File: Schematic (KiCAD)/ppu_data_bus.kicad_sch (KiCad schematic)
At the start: 111 parts

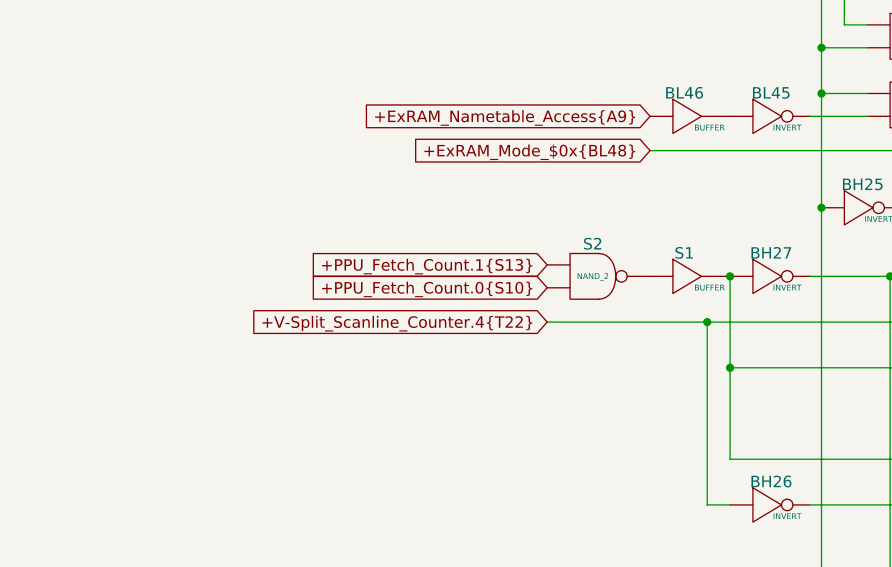
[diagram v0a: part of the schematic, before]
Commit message: Schematic and SVG Updates
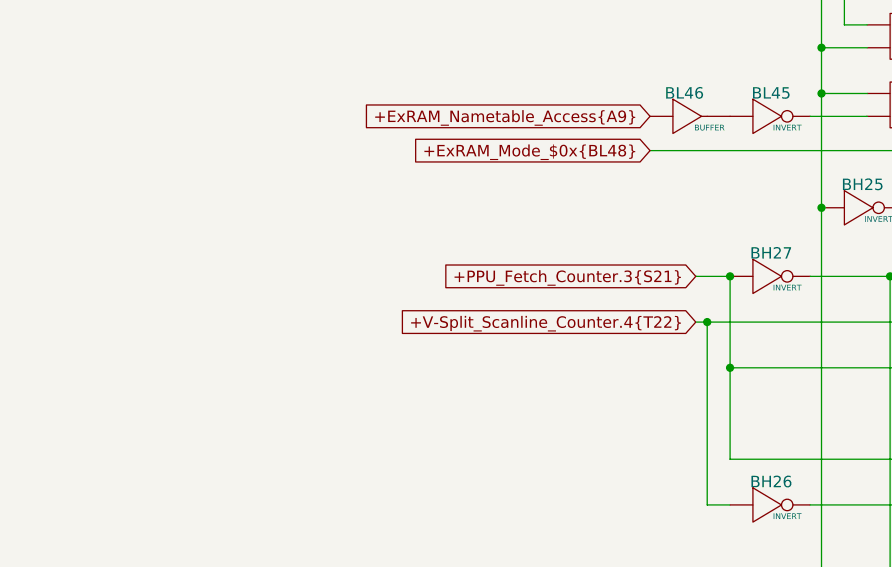
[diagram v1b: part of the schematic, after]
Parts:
- removed S1: BUFFER, symbol MMC5:BUFFER
- removed S2: NAND_2, symbol MMC5:NAND_2
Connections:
- net at BK24. (X): now also BK23. (X); no longer BK25. (X)
- net at BK23. (X): now also BL16. (X); no longer BK24. (X)
- net at BL14. (X): now also BL2. (X); no longer BK15. (X)
- net at BL45. (X): now also BL46. (X); no longer BL41. (X)
- net at BH21. (X): now also BH12. (X), BH4. (X); no longer BH22. (X)
- net at BK8. (X): now also BK7. (X); no longer BK9. (X)
- net at BK7. (X): now also BK15. (X), BK23. (X), BK31. (X), BK43. (X); no longer BK8. (X)
- net at BH19. (X): now also BH14. (X), BH6. (X); no longer BH20. (X)
- net at BH11. (X): now also BH12. (X); no longer BH13. (X)
- net at BL19. (X): now also BL7. (X); no longer BK35. (X)
- net at BL35. (X): now also BL29. (X); no longer BL40. (X)
- net at BL12. (X): now also BK1. (X); no longer BK7. (X)
- net at BK31. (X): now also BK32. (X); no longer BL18. (X)
- net at BK32. (X): now also BK33. (X); no longer BK31. (X)
- net at BK36. (X): now also BK35. (X); no longer BK37. (X)
- net at BH18. (X): now also BH22. (X), BH27. (X); no longer BH17. (X)
- net at BK28. (X): now also BK27. (X); no longer BK29. (X)
- net at BH2. (X): now also BH3. (X); no longer BH1. (X)
- net at BH3. (X): now also BH6. (X); no longer BH2. (X)
- net at BL16. (X): now also BL4. (X); no longer BK23. (X)
- net at BK11. (X): now also BK12. (X); no longer BL13. (X)
- net at BK12. (X): now also BK13. (X); no longer BK11. (X)
- net at BH10. (X): now also BH11. (X); no longer BH9. (X)
- net at BL15. (X): now also BK19. (X); no longer BL3. (X)
- net at BL17. (X): now also BL5. (X); no longer BK27. (X)
- net +PPU_Fetch_Counter.3{S21}: now reaches BH20. (X), BH24. (X), BH27. (X)
- net at BL37. (X): now also BL38. (X), BL42. (X); no longer BL36. (X)
- net at BK20. (X): now also BK19. (X); no longer BK21. (X)
- new net: BK24. (X), BK25. (X)
- new net: BL12. (X), BL13. (X), BL14. (X), BL15. (X), BL16. (X), BL17. (X), BL18. (X), BL19. (X), BL31. (X)
- new net: BK15. (X), BL14. (X)
- new net: BK10. (X), BK14. (X), BK18. (X), BK22. (X), BK26. (X), BK30. (X), BK34. (X), BK38. (X), BL39. (X)
- new net: BL41. (X), BL45. (X)
- new net: BL41. (X), BL42. (X)
- new net: BH21. (X), BH22. (X)
- new net: BK8. (X), BK9. (X)
- new net: BH19. (X), BH20. (X)
- new net: BK25. (X), BK26. (X)
- new net: BH13. (X), BH23. (X), BH5. (X)
- new net: BH11. (X), BH13. (X)
- new net: BK35. (X), BL19. (X)
- new net: BK10. (X), BK9. (X)
- new net: BL34. (X), BL35. (X), BL37. (X)
- new net: BL35. (X), BL40. (X)
- new net: BK7. (X), BL12. (X)
- new net: BK15. (X), BK23. (X), BK31. (X), BK42. (X), BK7. (X)
- new net: BK31. (X), BL18. (X)
- new net: BK37. (X), BK38. (X)
- new net: BK36. (X), BK37. (X)
- new net: BH18. (X), BH20. (X), BH26. (X)
- new net: BH18. (X), BH20. (X), BH22. (X), BH24. (X), BH25. (X)
- new net: BH17. (X), BH18. (X)
- new net: BH15. (X), BH17. (X), BH7. (X)
- new net: BH11. (X), BH15. (X)
- new net: BK29. (X), BK30. (X)
- new net: BK28. (X), BK29. (X)
- new net: BK11. (X), BK19. (X), BK27. (X), BK35. (X), BK40. (X)
- new net: BK39. (X), BK40. (X), BK42. (X)
- new net: BH1. (X), BH2. (X)
- new net: BK11. (X), BK19. (X), BK27. (X), BK35. (X), BK41. (X)
- new net: BK11. (X), BL13. (X)
- new net: BK21. (X), BK22. (X)
- new net: BK13. (X), BK14. (X)
- new net: BH10. (X), BH9. (X)
- new net: BK4. (X), BK5. (X)
- new net: BK2. (X), BK5. (X)
- new net: BL28. (X), BL29. (X), BL37. (X)
- new net: BL15. (X), BL3. (X)
- new net: BK27. (X), BL17. (X)
- new net: BK41. (X), BK43. (X), BK44. (X)
- new net: BL36. (X), BL37. (X)
- new net: BK20. (X), BK21. (X)
- new net: BK33. (X), BK34. (X)
- new net: BH11. (X), BH16. (X)
- new net: BH3. (X), BH5. (X)
- new net: BH3. (X), BH8. (X)
- new net: BH3. (X), BH4. (X)
- new net: BH3. (X), BH7. (X)
- new net: BK17. (X), BK18. (X)
- new net: BH11. (X), BH14. (X)
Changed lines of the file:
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@@
 	)
 	(junction
+		(at 170.18 86.36)
+		(diameter 0)
+		(color 0 0 0 0)
+	)
+	(junction
 		(at 224.79 86.36)
 		(diameter 0)
@@
 	)
 	(junction
-		(at 170.18 86.36)
-		(diameter 0)
-		(color 0 0 0 0)
-	)
-	(junction
 		(at 345.44 120.65)
 		(diameter 0)
@@
 	(wire
 		(pts
+			(xy 166.37 86.36) (xy 170.18 86.36)
+		)
+		(stroke
+			(width 0)
+			(type default)
+		)
+	)
+	(wire
+		(pts
 			(xy 271.78 25.4) (xy 274.32 25.4)
 		)
@@
 	(wire
 		(pts
-			(xy 149.86 91.44) (xy 167.64 91.44)
+			(xy 166.37 91.44) (xy 167.64 91.44)
 		)
 		(stroke
@@
 		)
 	)
-	(global_label "+PPU_Fetch_Count.0{S10}"
-		(shape input)
-		(at 149.86 87.63 180)
-		(fields_autoplaced yes)
-		(effects
-			(font
-				(size 1.27 1.27)
-			)
-			(justify right)
-		)
-		(property "Intersheetrefs" "${INTERSHEET_REFS}"
-			(at 121.7773 87.63 0)
-			(effects
-				(font
-					(size 1.27 1.27)
-				)
-				(justify right)
-				(hide yes)
-			)
-		)
-	)
 	(global_label "PPU_D7_In{BigBuf}"
 		(shape output)
@@
 	(global_label "+V-Split_Scanline_Counter.4{T22}"
 		(shape input)
-		(at 149.86 91.44 180)
+		(at 166.37 91.44 180)
 		(fields_autoplaced yes)
 		(effects
@@
 		)
 		(property "Intersheetrefs" "${INTERSHEET_REFS}"
-			(at 114.0365 91.44 0)
+			(at 130.5465 91.44 0)
 			(effects
 				(font
@@
 		)
 	)
-	(global_label "+PPU_Fetch_Count.1{S13}"
-		(shape input)
-		(at 149.86 85.09 180)
-		(fields_autoplaced yes)
-		(effects
-			(font
-				(size 1.27 1.27)
-			)
-			(justify right)
-		)
-		(property "Intersheetrefs" "${INTERSHEET_REFS}"
-			(at 121.7773 85.09 0)
-			(effects
-				(font
-					(size 1.27 1.27)
-				)
-				(justify right)
-				(hide yes)
-			)
-		)
-	)
 	(global_label "PPU_D0_IN_PIN"
 		(shape input)
@@
 		)
 	)
+	(global_label "+PPU_Fetch_Counter.3{S21}"
+		(shape input)
+		(at 166.37 86.36 180)
+		(fields_autoplaced yes)
+		(effects
+			(font
+				(size 1.27 1.27)
+			)
+			(justify right)
+		)
+		(property "Intersheetrefs" "${INTERSHEET_REFS}"
+			(at 136.4125 86.36 0)
+			(effects
+				(font
+					(size 1.27 1.27)
+				)
+				(justify right)
+				(hide yes)
+			)
+		)
+	)
 	(global_label "+$5106.5_Fill_Mode_Tile{L17}"
 		(shape input)
@@
 	)
 	(symbol
-		(lib_name "NAND_2_45")
-		(lib_id "MMC5:NAND_2")
-		(at 154.94 86.36 0)
-		(unit 1)
-		(exclude_from_sim no)
-		(in_bom yes)
-		(on_board yes)
-		(dnp no)
-		(fields_autoplaced yes)
-		(property "Reference" "S2"
-			(at 154.94 82.042 0)
-			(do_not_autoplace yes)
-			(effects
-				(font
-					(size 1.27 1.27)
-				)
-				(justify top)
-			)
-		)
-		(property "Value" "NAND_2"
-			(at 154.94 86.36 0)
-			(do_not_autoplace yes)
-			(effects
-				(font
-					(size 0.635 0.635)
-				)
-			)
-		)
-		(property "Footprint" ""
-			(at 154.94 86.36 0)
-			(effects
-				(font
-					(size 1.27 1.27)
-				)
-				(hide yes)
-			)
-		)
-		(property "Datasheet" ""
-			(at 154.94 86.36 0)
-			(effects
-				(font
-					(size 1.27 1.27)
-				)
-				(hide yes)
-			)
-		)
-		(property "Description" ""
-			(at 154.94 86.36 0)
-			(effects
-				(font
-					(size 1.27 1.27)
-				)
-				(hide yes)
-			)
-		)
-		(pin ""
-		)
-		(pin ""
-		)
-		(pin ""
-		)
-		(instances
-			(project "MMC5"
-				(path "/46093bf6-f83e-4237-9ece-7350a682aff0/4e6a5c22-b922-467f-8545-4eb558480830"
-					(reference "S2")
-					(unit 1)
-				)
-			)
-		)
-	)
-	(symbol
 		(lib_name "NAND_3_4")
 		(lib_id "MMC5:NAND_3")
@@
 					(unit 1)
 				)
-			)
-		)
-	)
-	(symbol
-		(lib_name "BUFFER_29")
-		(lib_id "MMC5:BUFFER")
-		(at 165.1 86.36 0)
-		(unit 1)
-		(exclude_from_sim no)
-		(in_bom yes)
-		(on_board yes)
-		(dnp no)
-		(fields_autoplaced yes)
-		(property "Reference" "S1"
-			(at 165.1 83.058 0)
-			(do_not_autoplace yes)
-			(effects
-				(font
-					(size 1.27 1.27)
-				)
-				(justify top)
-			)
-		)
-		(property "Value" "BUFFER"
-			(at 167.894 87.63 0)
-			(do_not_autoplace yes)
-			(effects
-				(font
-					(size 0.635 0.635)
-				)
-			)
-		)
-		(property "Footprint" ""
-			(at 165.1 86.36 0)
-			(effects
-				(font
-					(size 1.27 1.27)
-				)
-				(hide yes)
-			)
-		)
-		(property "Datasheet" ""
-			(at 165.1 86.36 0)
-			(effects
-				(font
-					(size 1.27 1.27)
-				)
-				(hide yes)
-			)
-		)
-		(property "Description" ""
-			(at 165.1 86.36 0)
-			(effects
-				(font
-					(size 1.27 1.27)
-				)
-				(hide yes)
-			)
-		)
-		(pin ""
-		)
-		(pin ""
-		)
-		(instances
-			(project "MMC5"
-				(path "/46093bf6-f83e-4237-9ece-7350a682aff0/4e6a5c22-b922-467f-8545-4eb558480830"
-					(reference "S1")
-					(unit 1)
-				)
